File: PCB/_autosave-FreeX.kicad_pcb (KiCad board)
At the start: 2 copper layers, 40 parts, among them J1 2-1734839-4, J2 TF31-6S-0.5SH_800_, J3 USB4105-GF-A, J4 TF31-6S-0.5SH_800_, J5 TF31-6S-0.5SH_800_, Q1 BC817, Q2 BC817, U1 W25Q32JVZPIQ, U2 MPU-9250, U3 ESP32-D0WDQ6, U4 CP2102, U5 TC2014-3.3VxCTTR, U6 LM358PW, U7 TDA7052AT_N2, Y1 ECS-400-10-36-CKY-TR

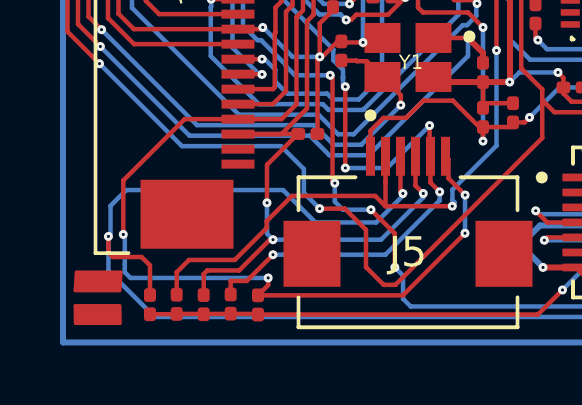
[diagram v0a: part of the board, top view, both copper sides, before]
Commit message: 15th, march. 2025
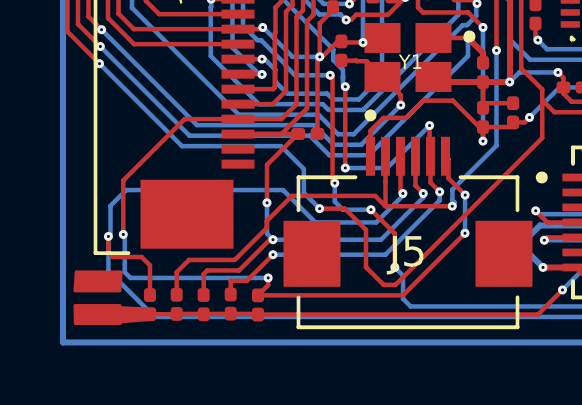
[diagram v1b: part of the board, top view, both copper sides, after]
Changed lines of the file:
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@@
+	(gr_poly
+		(pts
+			(xy 78.155425 43.38) (xy 79.51 43.44) (xy 79.49 43.68) (xy 78.095425 43.789809) (xy 78.125425 43.389809)
+			(xy 78.145425 43.429809) (xy 78.205425 43.409809) (xy 78.175425 43.409809)
+		)
+		(stroke
+			(width 0.2)
+			(type solid)
+		)
+		(fill solid)
+		(layer "F.Cu")
+		(net 140)
+	)
 	(gr_poly
 		(pts
